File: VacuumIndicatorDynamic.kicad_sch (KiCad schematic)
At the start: 50 parts, among them J1 Conn_01x02_Male, J2 Conn_01x03_Male, J3 Conn_01x03_Male, J4 Conn_01x03_Male, SW1 SW_DIP_x01, SW2 SW_DIP_x01, SW3 SW_DIP_x01, SW4 SW_DIP_x01, U1 AP1117-25, U2 YAAJ_BluePill

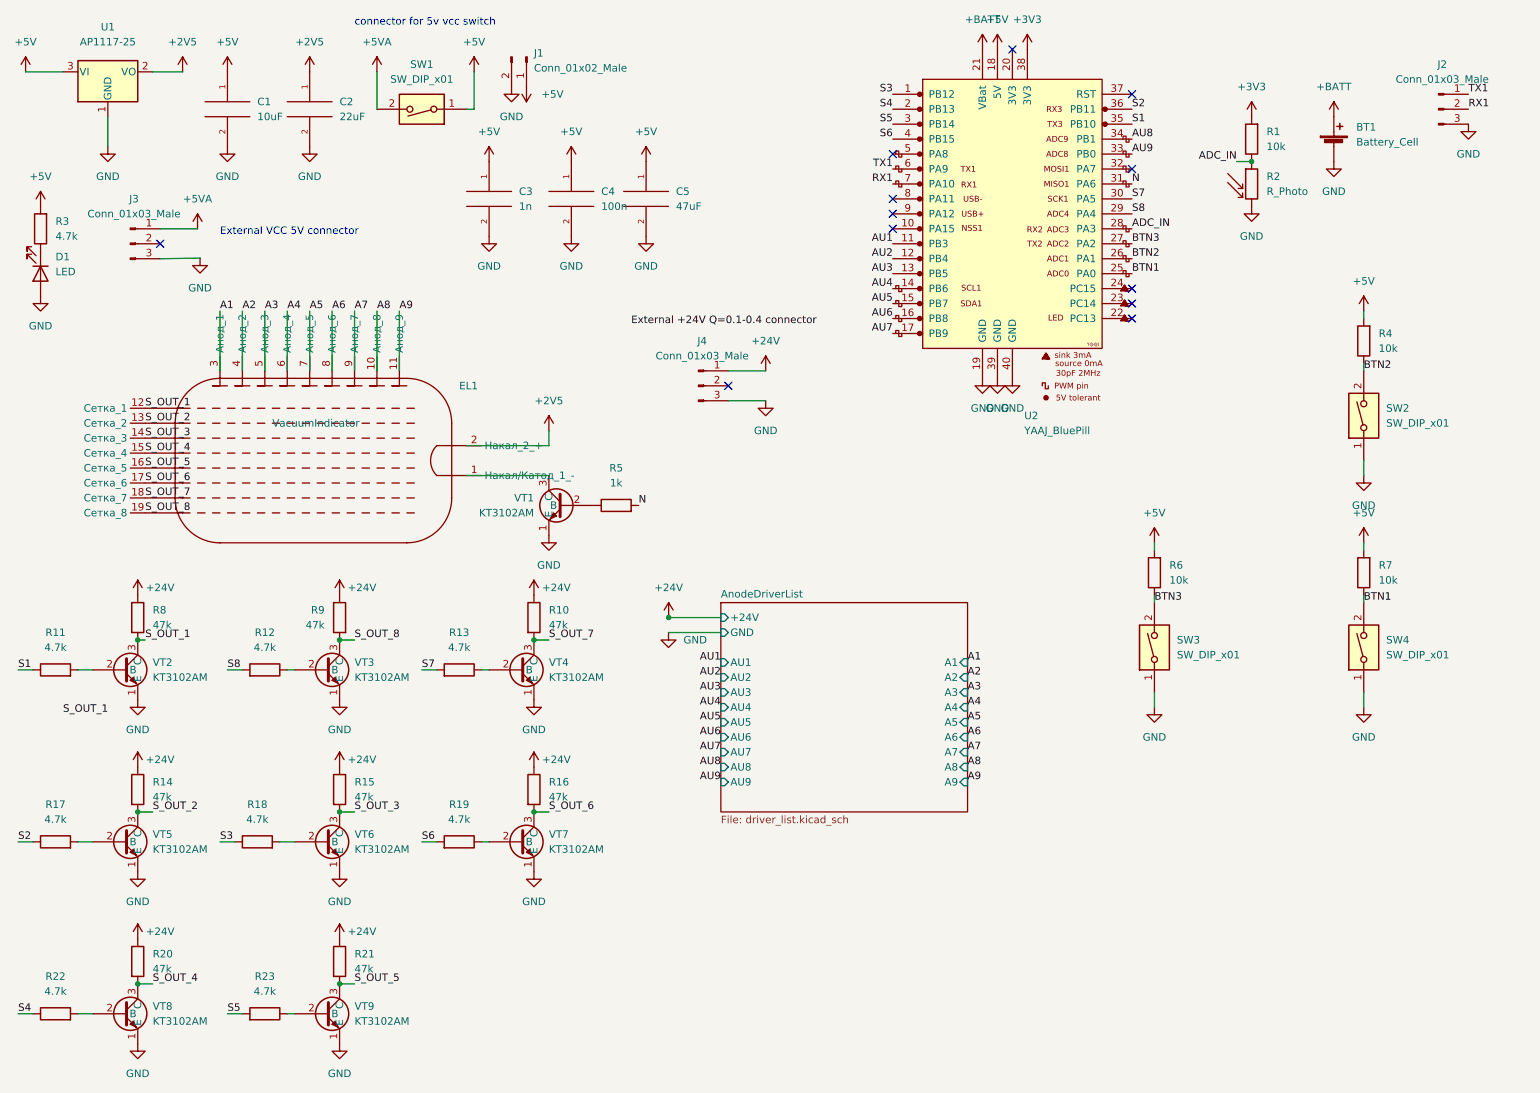
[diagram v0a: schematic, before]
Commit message: Remake sch after fabrication. Clear repo
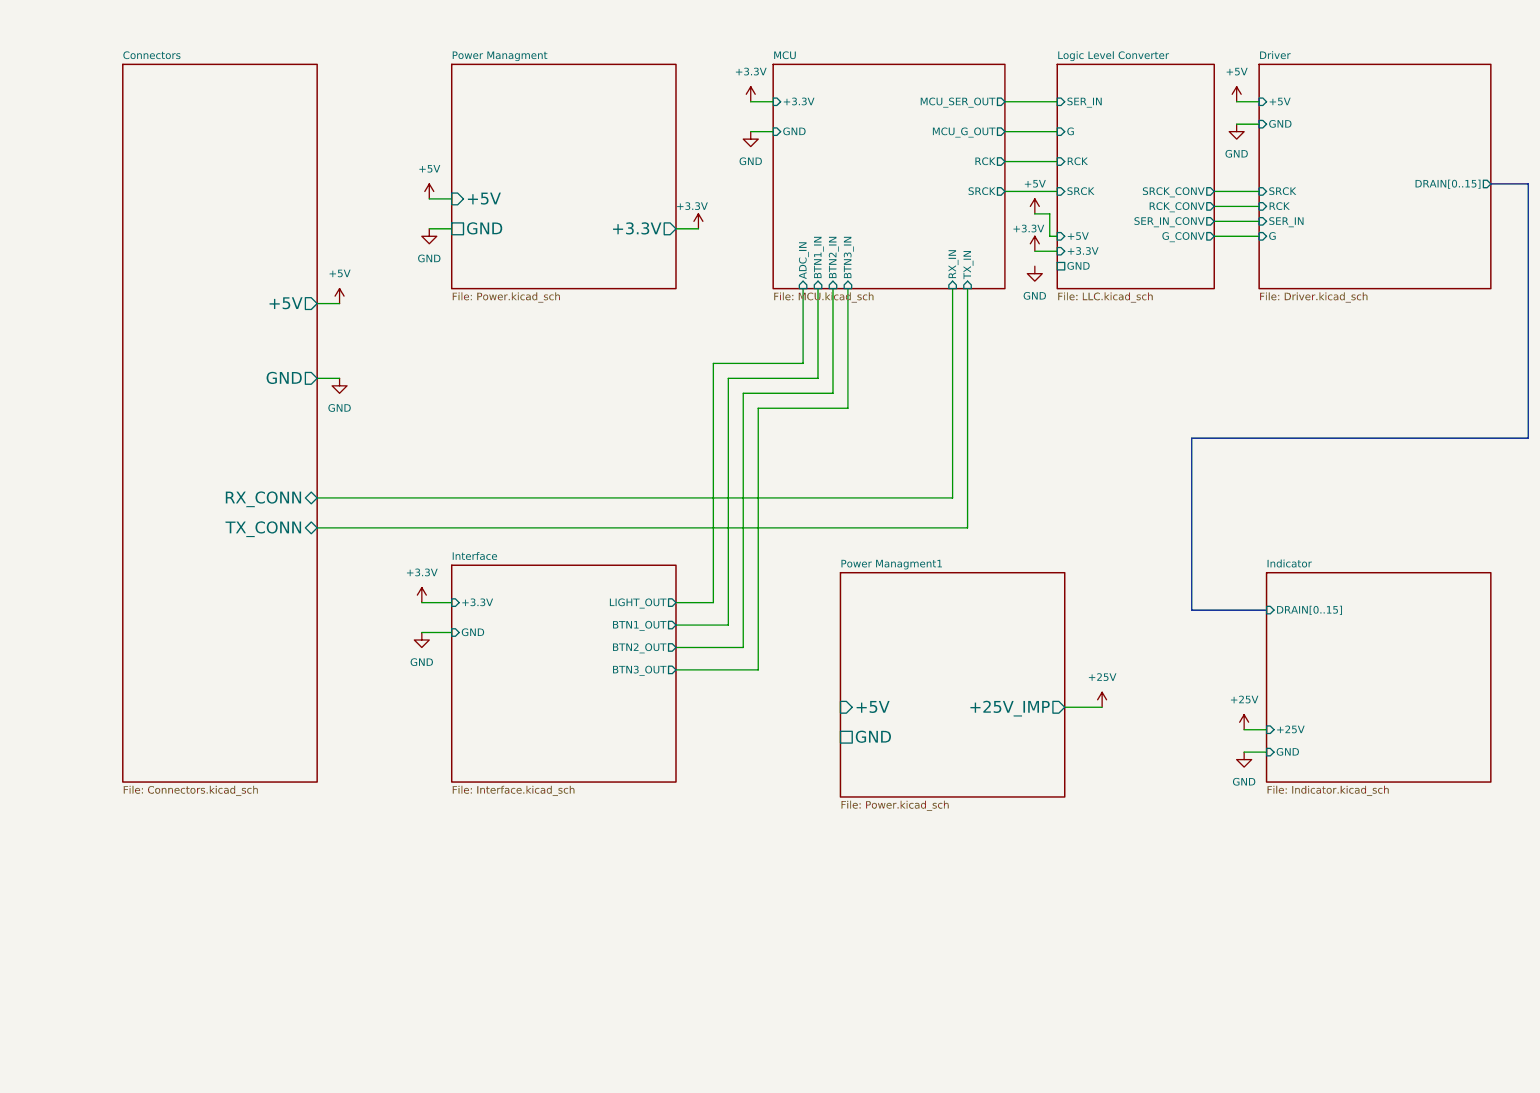
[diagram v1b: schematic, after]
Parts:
- removed BT1: Battery_Cell, Connector_PinHeader_2.54mm:PinHeader_1x02_P2.54mm_Vertical, symbol Device:Battery_Cell
- removed C1: 10uF, Capacitor_THT:CP_Radial_D6.3mm_P2.50mm, symbol pspice:CAP
- removed C2: 22uF, Capacitor_THT:CP_Radial_D6.3mm_P2.50mm, symbol pspice:CAP
- removed C3: 1n, Capacitor_SMD:C_0805_2012Metric, symbol pspice:CAP
- removed C4: 100n, Capacitor_SMD:C_0805_2012Metric, symbol pspice:CAP
- removed C5: 47uF, Capacitor_THT:CP_Radial_D8.0mm_P5.00mm, symbol pspice:CAP
- removed D1: LED, LED_SMD:LED_0805_2012Metric, symbol Device:LED
- removed EL1: VacuumIndicator, ProjectLibrary:VauumIndicator_ILC_8-9, symbol ProjectLib:VacuumIndicator
- removed J1: Conn_01x02_Male, Connector_PinHeader_2.54mm:PinHeader_1x02_P2.54mm_Vertical, symbol Connector:Conn_01x02_Male
- removed J2, J3, J4: Conn_01x03_Male, Connector_PinHeader_2.54mm:PinHeader_1x03_P2.54mm_Vertical, symbol Connector:Conn_01x03_Male
- removed R1, R4, R6, R7: 10k, Resistor_SMD:R_0805_2012Metric, symbol Device:R
- removed R10, R14, R15, R16, R20, R21, R8, R9: 47k, Resistor_SMD:R_0805_2012Metric, symbol Device:R
- removed R11, R12, R13, R17, R18, R19, R22, R23, R3: 4.7k, Resistor_SMD:R_0805_2012Metric, symbol Device:R
- removed R2: R_Photo, Resistor_THT:R_Axial_DIN0204_L3.6mm_D1.6mm_P1.90mm_Vertical, symbol Device:R_Photo
- removed R5: 1k, Resistor_SMD:R_0805_2012Metric, symbol Device:R
- removed SW1: SW_DIP_x01, Connector_PinSocket_2.54mm:PinSocket_1x02_P2.54mm_Vertical, symbol Switch:SW_DIP_x01
- removed SW2, SW3, SW4: SW_DIP_x01, Button_Switch_SMD:SW_SPST_FSMSM, symbol Switch:SW_DIP_x01
- removed U1: AP1117-25, Package_TO_SOT_SMD:SOT-223-3_TabPin2, symbol Regulator_Linear:AP1117-25
- removed U2: YAAJ_BluePill, ProjectLibrary:YAAJ_BluePill_1, symbol ProjectLib:YAAJ_BluePill
- removed VT1, VT2, VT3, VT4, VT5, VT6, VT7, VT8, VT9: KT3102AM, Package_TO_SOT_THT:TO-92_HandSolder, symbol ProjectLib:KT3102AM
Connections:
- no-connect marks 12 -> 0
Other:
- removed sheet AnodeDriverList
- added sheet Connectors (Connectors.kicad_sch)
- added sheet Driver (Driver.kicad_sch)
- added sheet Indicator (Indicator.kicad_sch)
- added sheet Interface (Interface.kicad_sch)
- added sheet Logic Level Converter (LLC.kicad_sch)
- added sheet MCU (MCU.kicad_sch)
- added sheet Power Managment (Power.kicad_sch)
- added sheet Power Managment1 (Power.kicad_sch)
- note removed: "External VCC 5V connector"
- note removed: "connector for 5v vcc switch"
